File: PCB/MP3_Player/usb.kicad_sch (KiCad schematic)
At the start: 13 parts, among them J2 USB_C_Receptacle_16P, J3 USB_A, U4 TS3USB30ERSWR

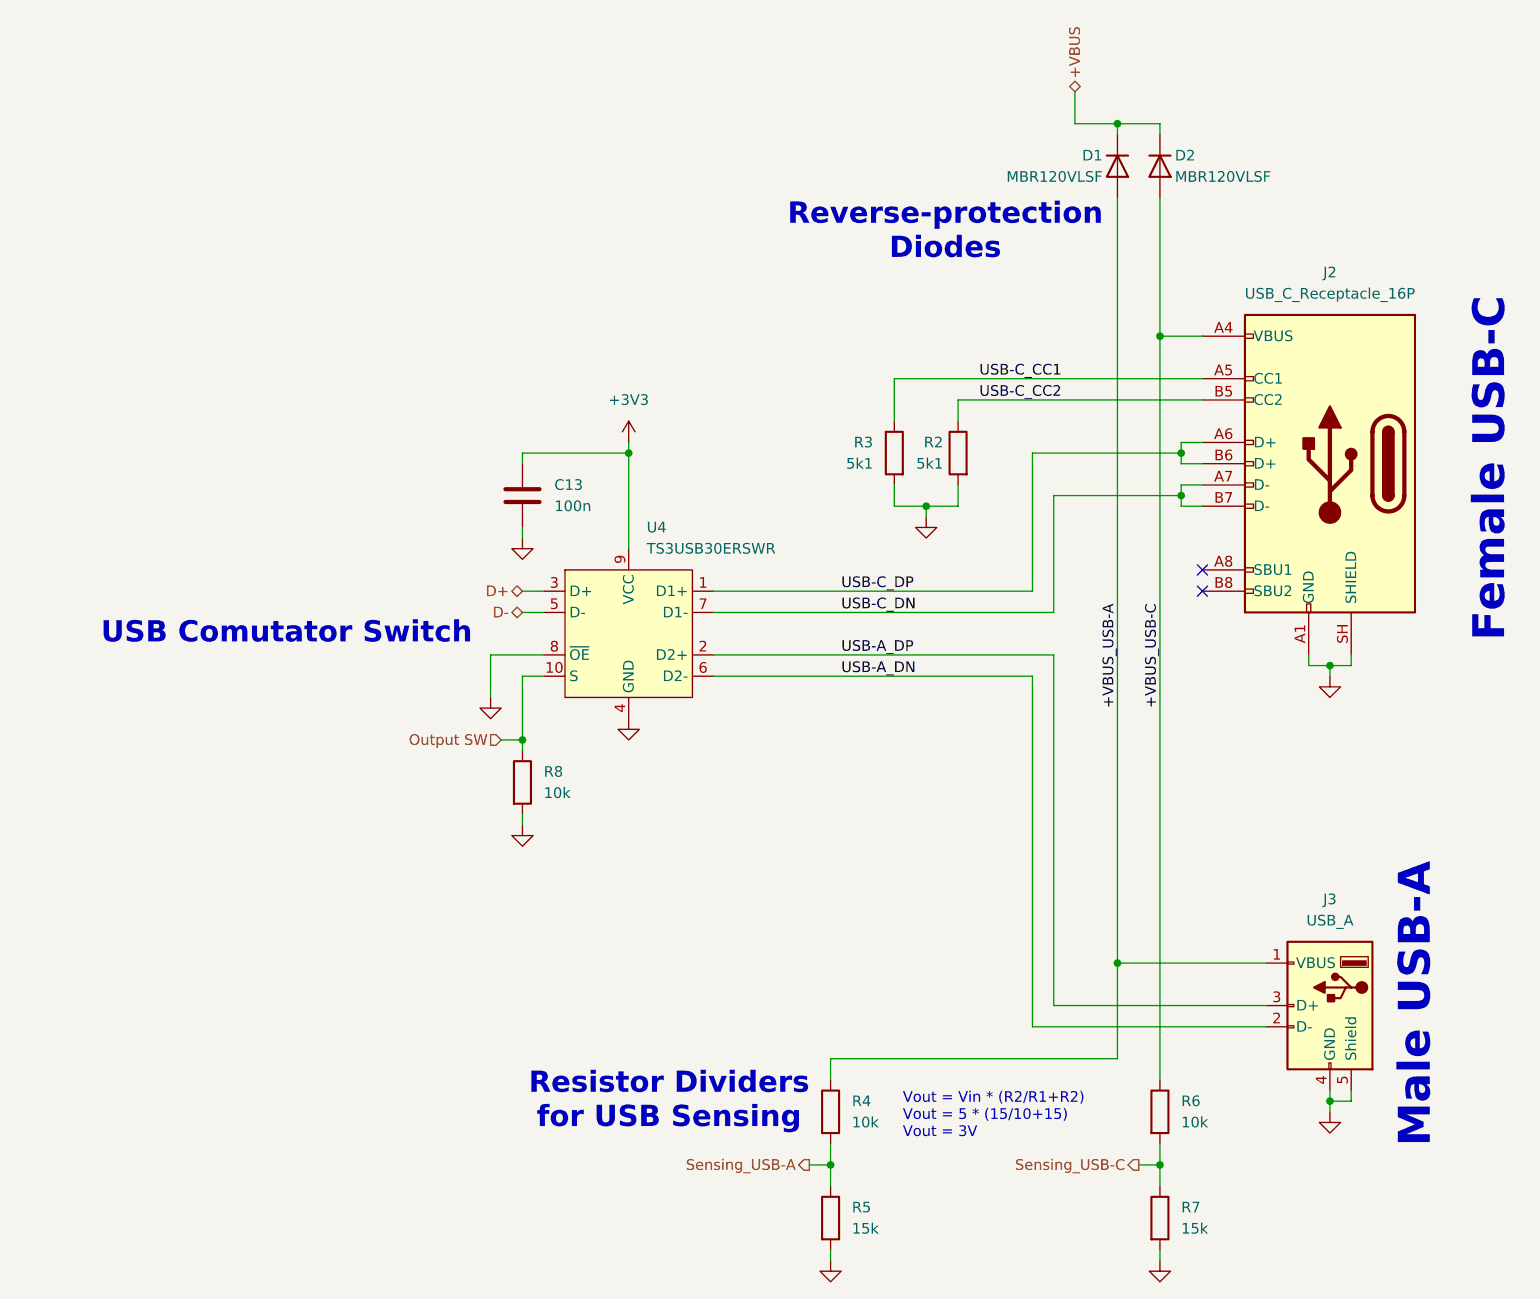
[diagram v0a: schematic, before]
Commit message: PCB Routing
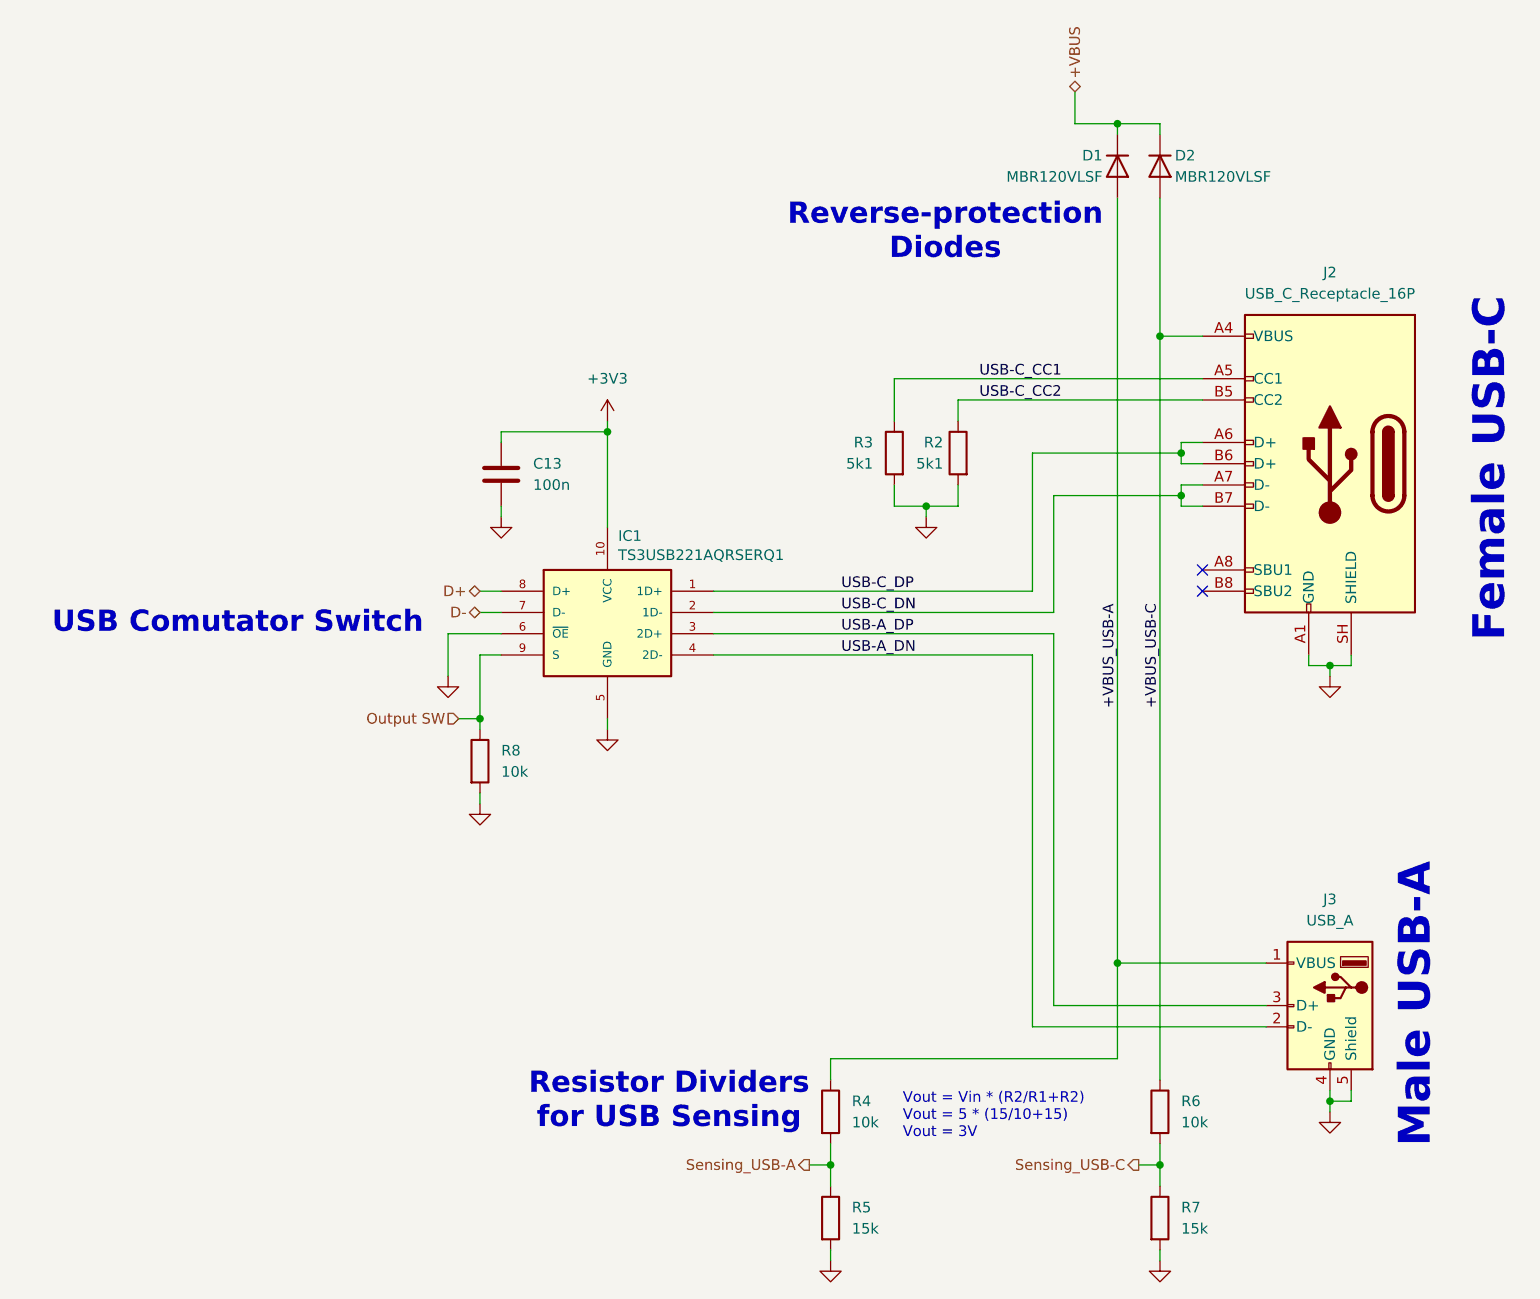
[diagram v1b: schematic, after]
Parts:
- removed U4: TS3USB30ERSWR, Package_DFN_QFN:UQFN-10_1.4x1.8mm_P0.4mm, symbol Interface_USB:TS3USB30ERSWR
- added IC1: TS3USB221AQRSERQ1, TS3USB221AQRSERQ1:TS3USB221AQRSERQ1, symbol TS3USB221AQRSERQ1:TS3USB221AQRSERQ1
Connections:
- net +3V3: now also IC1.10 (VCC)
- net D+: now also IC1.8 (D+)
- net D-: now also IC1.7 (D-)
- net GND: now also IC1.5 (GND), IC1.6 (~{OE})
- net Output SW: now also IC1.9 (S)
- net USB-A_DN: now also IC1.4 (2D-)
- net USB-A_DP: now also IC1.3 (2D+)
- net USB-C_DN: now also IC1.2 (1D-)
- net USB-C_DP: now also IC1.1 (1D+)
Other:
- moved on the sheet: C13, R8
